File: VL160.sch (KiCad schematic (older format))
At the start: 15 parts, among them J1 USB_C_Receptacle, J2 USB3_A, U1 VL160, U2 SE8550

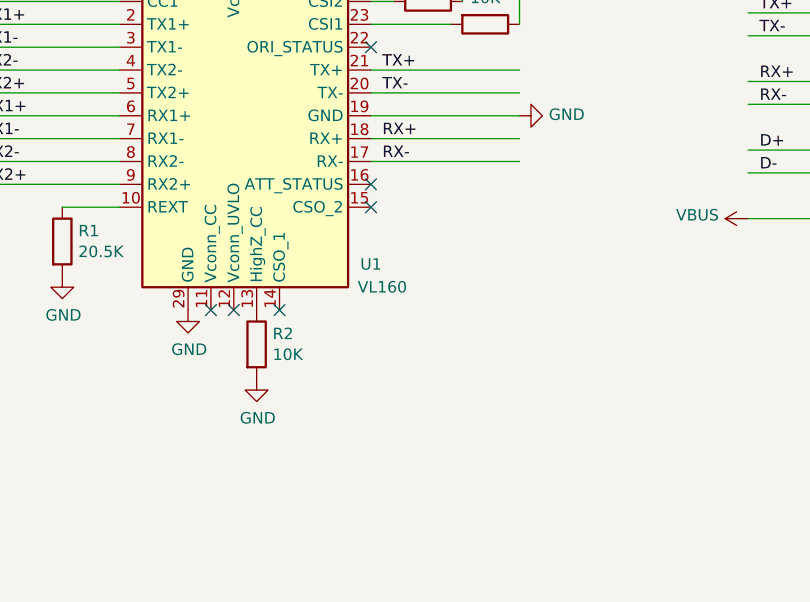
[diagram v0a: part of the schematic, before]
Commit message: Sync 2022/01/19 周三 11:41:49.34
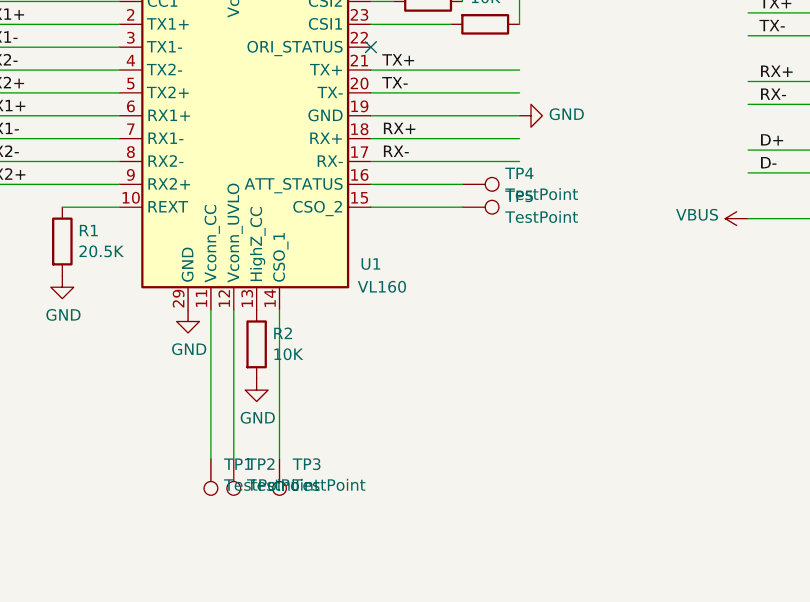
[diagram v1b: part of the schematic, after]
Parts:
- added TP1, TP2, TP3, TP4, TP5: TestPoint, VL160:TestPoint_Pad_D0.7mm, symbol Connector:TestPoint
- J1: footprint VL160:USB-C-SMD_TYPE-C-31-G-01 -> Connector_USB:USB_C_Receptacle_Amphenol_12401548E4-2A
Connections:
- wire segments 55 -> 60
- no-connect marks 8 -> 3
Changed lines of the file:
@@
 F 0 "J1" H 2507 4217 50  0000 C CNN
 F 1 "USB_C_Receptacle" H 2507 4126 50  0000 C CNN
-F 2 "VL160:USB-C-SMD_TYPE-C-31-G-01" H 2550 2950 50  0001 C CNN
+F 2 "Connector_USB:USB_C_Receptacle_Amphenol_12401548E4-2A" H 2550 2950 50  0001 C CNN
 F 3 "https://www.usb.org/sites/default/files/documents/usb_type-c.zip" H 2550 2950 50  0001 C CNN
 	1    2400 2950
@@
 	1    8750 3200
 	-1   0    0    1
-$EndComp
-$Comp
-L VL160:VL160 U1
-U 1 1 61D5D001
-P 5450 2700
-F 0 "U1" H 5950 1600 50  0000 C CNN
-F 1 "VL160" H 6000 1500 50  0000 C CNN
-F 2 "VL160:WQFN-28_L4.5-W3.5-H0.8-P0.4" H 3900 -200 50  0001 L CNN
-F 3 "https://www.silabs.com/documents/public/data-sheets/cp2102n-datasheet.pdf" H 5500 1950 50  0001 C CNN
-	1    5450 2700
-	1    0    0    -1
 $EndComp
 Wire Wire Line
@@
 	1    0    0    -1
 $EndComp
-NoConn ~ 5250 4000
-NoConn ~ 5350 4000
-NoConn ~ 5550 4000
-NoConn ~ 5950 3550
-NoConn ~ 5950 3450
 Wire Wire Line
 	7600 3400 8250 3400
@@
 	1    0    0    -1
 $EndComp
-Connection ~ 5450 2200
 Wire Wire Line
 	8750 2500 8850 2500
@@
 	1    0    0    -1
 $EndComp
+Connection ~ 5450 2200
+$Comp
+L VL160:VL160 U1
+U 1 1 61D5D001
+P 5450 2700
+F 0 "U1" H 5950 1600 50  0000 C CNN
+F 1 "VL160" H 6000 1500 50  0000 C CNN
+F 2 "VL160:WQFN-28_L4.5-W3.5-H0.8-P0.4" H 3900 -200 50  0001 L CNN
+F 3 "https://www.silabs.com/documents/public/data-sheets/cp2102n-datasheet.pdf" H 5500 1950 50  0001 C CNN
+	1    5450 2700
+	1    0    0    -1
+$EndComp
+$Comp
+L Connector:TestPoint TP1
+U 1 1 61E11662
+P 5250 4650
+F 0 "TP1" H 5192 4676 50  0000 R CNN
+F 1 "TestPoint" H 5192 4767 50  0000 R CNN
+F 2 "VL160:TestPoint_Pad_D0.7mm" H 5450 4650 50  0001 C CNN
+F 3 "~" H 5450 4650 50  0001 C CNN
+	1    5250 4650
+	-1   0    0    1
+$EndComp
+$Comp
+L Connector:TestPoint TP2
+U 1 1 61E1235A
+P 5350 4650
+F 0 "TP2" H 5292 4676 50  0000 R CNN
+F 1 "TestPoint" H 5292 4767 50  0000 R CNN
+F 2 "VL160:TestPoint_Pad_D0.7mm" H 5550 4650 50  0001 C CNN
+F 3 "~" H 5550 4650 50  0001 C CNN
+	1    5350 4650
+	-1   0    0    1
+$EndComp
+$Comp
+L Connector:TestPoint TP3
+U 1 1 61E126B1
+P 5550 4650
+F 0 "TP3" H 5492 4676 50  0000 R CNN
+F 1 "TestPoint" H 5492 4767 50  0000 R CNN
+F 2 "VL160:TestPoint_Pad_D0.7mm" H 5750 4650 50  0001 C CNN
+F 3 "~" H 5750 4650 50  0001 C CNN
+	1    5550 4650
+	-1   0    0    1
+$EndComp
+$Comp
+L Connector:TestPoint TP5
+U 1 1 61E1285F
+P 6350 3550
+F 0 "TP5" V 6304 3738 50  0000 L CNN
+F 1 "TestPoint" V 6395 3738 50  0000 L CNN
+F 2 "VL160:TestPoint_Pad_D0.7mm" H 6550 3550 50  0001 C CNN
+F 3 "~" H 6550 3550 50  0001 C CNN
+	1    6350 3550
+	0    1    1    0
+$EndComp
+$Comp
+L Connector:TestPoint TP4
+U 1 1 61E12E64
+P 6350 3450
+F 0 "TP4" V 6304 3638 50  0000 L CNN
+F 1 "TestPoint" V 6395 3638 50  0000 L CNN
+F 2 "VL160:TestPoint_Pad_D0.7mm" H 6550 3450 50  0001 C CNN
+F 3 "~" H 6550 3450 50  0001 C CNN
+	1    6350 3450
+	0    1    1    0
+$EndComp
+Wire Wire Line
+	5250 4000 5250 4650
+Wire Wire Line
+	5350 4650 5350 4000
+Wire Wire Line
+	5550 4000 5550 4650
+Wire Wire Line
+	5950 3450 6350 3450
+Wire Wire Line
+	6350 3550 5950 3550
 $EndSCHEMATC
